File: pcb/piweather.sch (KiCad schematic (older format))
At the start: 60 parts, among them J1 Screw_Terminal_01x10, J10 Conn_01x03_Male, J11 Conn_01x03_Male, J12 Conn_01x02_Male, J2 Conn_01x08_Male, J3 Screw_Terminal_01x02, J4 Raspberry_Pi_2_3, J5 Conn_01x03_Male, J6 Conn_01x01_Male, J7 Conn_01x01_Male, J8 Conn_01x01_Male, J9 Conn_01x01_Male, Q1 2N7002, Q2 2N7002, U1 FT2232D, U2 PSK-S5B-5, U3 THVD1500, U4 V78E05-1000-SMT-TR, U5 Si7020-A20, U6 TLV61046ADB, U7 74HC14, U8 LM339, Y1 Resonator

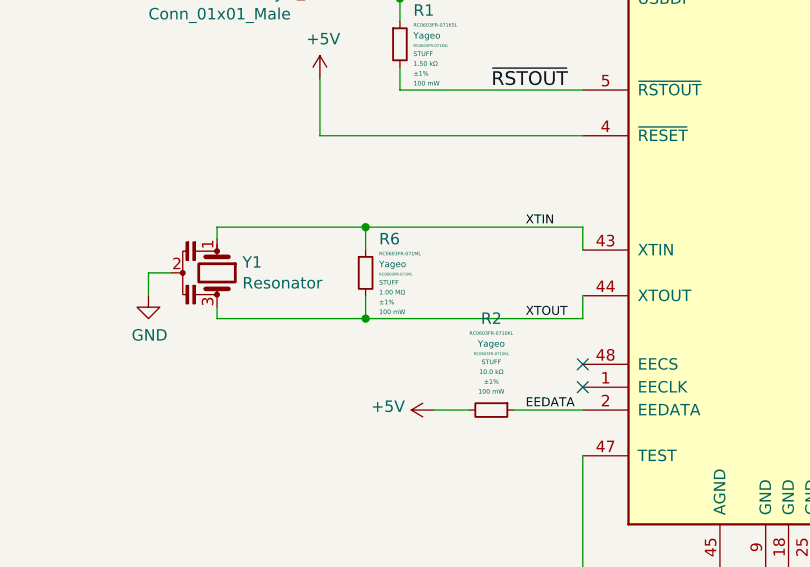
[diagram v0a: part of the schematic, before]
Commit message: layout in progress
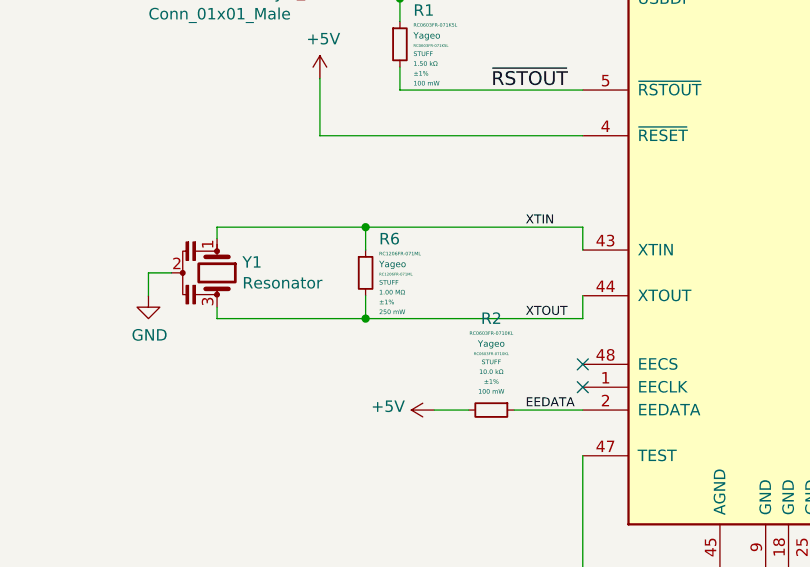
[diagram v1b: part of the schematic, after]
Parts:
- removed R6: RC0603FR-071ML, Main:RESC0603, symbol res_smd:RC0603FR-071ML
- added R6: RC1206FR-071ML, Main:RESC1206, symbol res_smd:RC1206FR-071ML
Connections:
- net XTIN: now also R6.1
- net XTOUT: now also R6.2
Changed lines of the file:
@@
 Wire Wire Line
 	1400 8000 1500 8000
-$Comp
-L res_smd:RC0603FR-071ML R6
-U 1 1 5DAEA189
-P 2350 8000
-F 0 "R6" H 2409 8148 50  0000 L CNN
-F 1 "RC0603FR-071ML" H 2409 8084 15  0000 L CNN
-F 2 "Main:RESC0603" H 2450 7925 10  0001 C CNN
-F 3 "" H 2380 8020 50  0000 C CNN
-F 4 "Yageo" H 2409 8038 28  0000 L CNN "Manufacturer"
-F 5 "RC0603FR-071ML" H 2409 7994 12  0000 L CNN "MPN"
-F 6 "STUFF" H 2409 7958 20  0000 L CNN "SKU"
-F 7 "1.00 MΩ" H 2409 7915 20  0000 L CNN "Res"
-F 8 "±1%" H 2409 7872 20  0000 L CNN "Tol"
-F 9 "100 mW" H 2409 7829 20  0000 L CNN "Pwr"
-	1    2350 8000
-	1    0    0    -1
-$EndComp
 Wire Wire Line
 	2350 7900 2350 7800
@@
 	1    0    0    -1
 $EndComp
+$Comp
+L res_smd:RC1206FR-071ML R6
+U 1 1 5DBA605D
+P 2350 8000
+F 0 "R6" H 2409 8148 50  0000 L CNN
+F 1 "RC1206FR-071ML" H 2409 8084 15  0000 L CNN
+F 2 "Main:RESC1206" H 2450 7925 10  0001 C CNN
+F 3 "" H 2380 8020 50  0000 C CNN
+F 4 "Yageo" H 2409 8038 28  0000 L CNN "Manufacturer"
+F 5 "RC1206FR-071ML" H 2409 7994 12  0000 L CNN "MPN"
+F 6 "STUFF" H 2409 7958 20  0000 L CNN "SKU"
+F 7 "1.00 MΩ" H 2409 7915 20  0000 L CNN "Res"
+F 8 "±1%" H 2409 7872 20  0000 L CNN "Tol"
+F 9 "250 mW" H 2409 7829 20  0000 L CNN "Pwr"
+	1    2350 8000
+	1    0    0    -1
+$EndComp
